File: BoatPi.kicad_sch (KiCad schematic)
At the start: 39 parts, among them J1 1432431, J2 1436987, J3 USB3_A_Stacked, J4 JAE_SIM_Card_SF72S006, J5 MDT420M01002, J6 G45A19071083HR, J7 1436987, J8 1432431, U1 SIM7600E-H, U2 PC817, U3 PC817, U4 PC817, U5 PC817, U6 PC817, U7 PC817, U8 PC817, U9 PC817

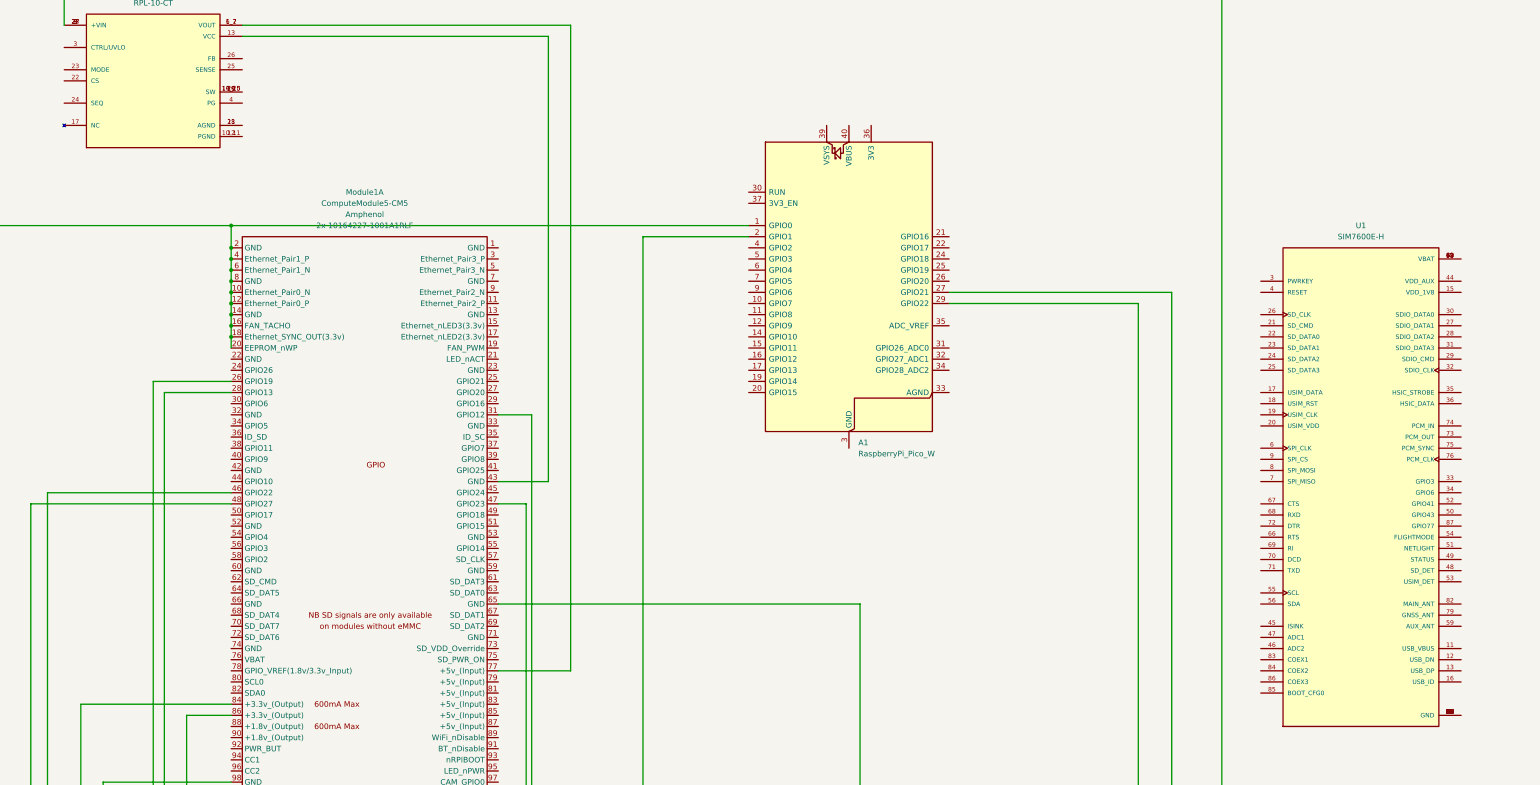
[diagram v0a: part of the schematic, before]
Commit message: Test Change
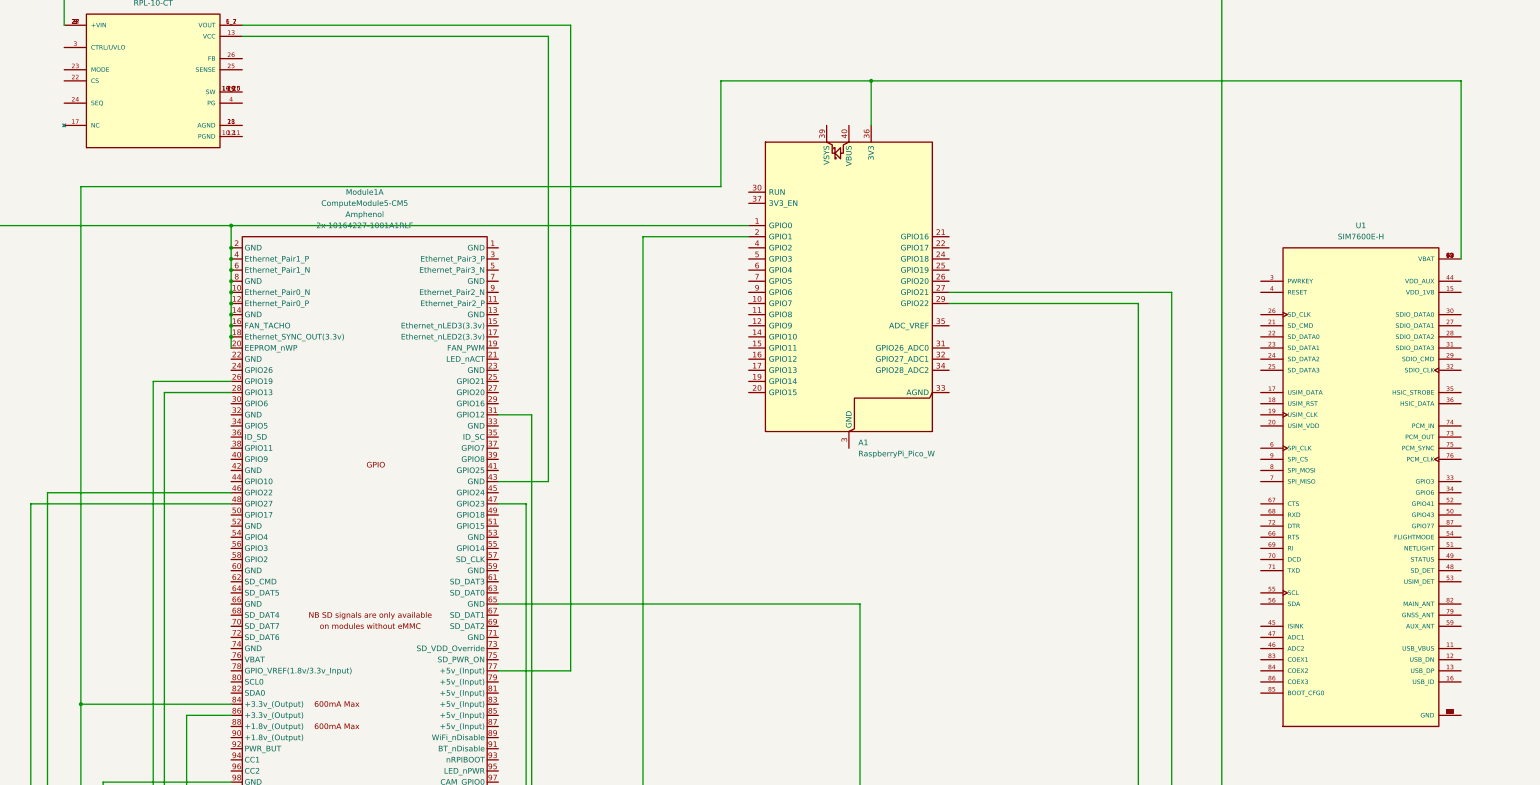
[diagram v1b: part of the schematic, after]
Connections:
- net at Module1.84 (+3.3v_(Output)), R11.1, R13.1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: now also A1.36 (3V3), U1.38 (VBAT), U1.39 (VBAT), U1.62 (VBAT), U1.63 (VBAT)
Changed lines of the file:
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@@
+	)
+	(junction
+		(at 39.37 274.32)
+		(diameter 0)
+		(color 0 0 0 0)
 	)
 	(junction
@@
 	)
 	(junction
+		(at 219.71 132.08)
+		(diameter 0)
+		(color 0 0 0 0)
+	)
+	(junction
 		(at 19.05 368.3)
 		(diameter 0)
@@
 	(wire
 		(pts
+			(xy 39.37 274.32) (xy 39.37 156.21)
+		)
+		(stroke
+			(width 0)
+			(type default)
+		)
+	)
+	(wire
+		(pts
 			(xy 217.17 330.2) (xy 217.17 331.47)
 		)
@@
 	(wire
 		(pts
+			(xy 39.37 156.21) (xy 185.42 156.21)
+		)
+		(stroke
+			(width 0)
+			(type default)
+		)
+	)
+	(wire
+		(pts
 			(xy 76.2 119.38) (xy 151.13 119.38)
 		)
@@
 	(wire
 		(pts
+			(xy 219.71 132.08) (xy 354.33 132.08)
+		)
+		(stroke
+			(width 0)
+			(type default)
+		)
+	)
+	(wire
+		(pts
 			(xy 177.8 372.11) (xy 177.8 328.93)
 		)
@@
 	(wire
 		(pts
+			(xy 185.42 132.08) (xy 219.71 132.08)
+		)
+		(stroke
+			(width 0)
+			(type default)
+		)
+	)
+	(wire
+		(pts
 			(xy 24.13 401.32) (xy 39.37 401.32)
 		)
@@
 	(wire
 		(pts
+			(xy 185.42 156.21) (xy 185.42 132.08)
+		)
+		(stroke
+			(width 0)
+			(type default)
+		)
+	)
+	(wire
+		(pts
 			(xy 77.47 354.33) (xy 58.42 354.33)
 		)
@@
 	(wire
 		(pts
+			(xy 354.33 172.72) (xy 354.33 132.08)
+		)
+		(stroke
+			(width 0)
+			(type default)
+		)
+	)
+	(wire
+		(pts
 			(xy 146.05 223.52) (xy 134.62 223.52)
 		)
@@
 		)
 		(stroke
+			(width 0)
+			(type default)
+		)
+	)
+	(wire
+		(pts
+			(xy 219.71 132.08) (xy 219.71 142.24)
+		)
+		(stroke

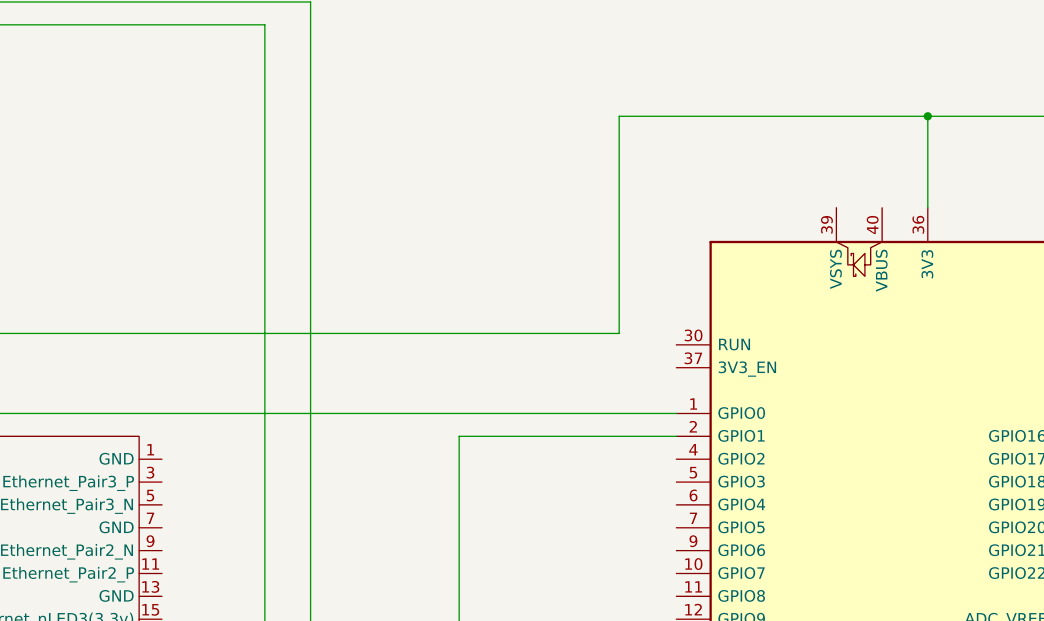
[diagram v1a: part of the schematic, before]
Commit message: New Test
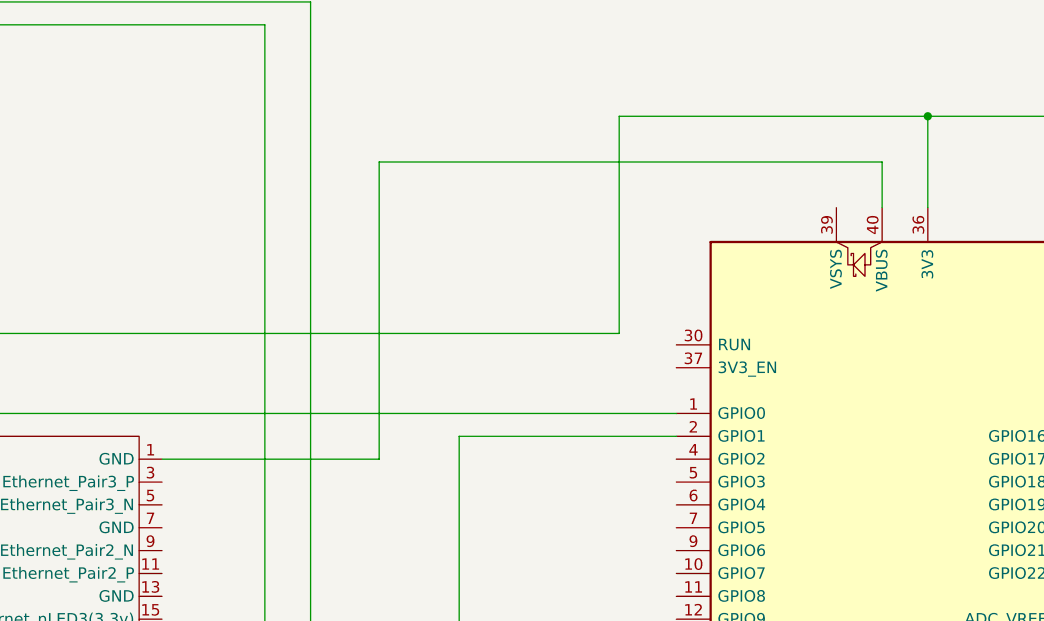
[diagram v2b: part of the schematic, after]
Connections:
- net at A1.40 (VBUS): now also Module1.1 (GND)
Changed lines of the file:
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@@
+	(wire
+		(pts
+			(xy 158.75 137.16) (xy 214.63 137.16)
+		)
+		(stroke
+			(width 0)
+			(type default)
+		)
+	)
 	(wire
 		(pts
@@
 	(wire
 		(pts
+			(xy 158.75 170.18) (xy 158.75 137.16)
+		)
+		(stroke
+			(width 0)
+			(type default)
+		)
+	)
+	(wire
+		(pts
 			(xy 55.88 200.66) (xy 55.88 332.74)
 		)
@@
 	(wire
 		(pts
+			(xy 214.63 137.16) (xy 214.63 142.24)
+		)
+		(stroke
+			(width 0)
+			(type default)
+		)
+	)
+	(wire
+		(pts
 			(xy 120.65 392.43) (xy 139.7 392.43)
 		)
@@
 		)
 		(stroke
+			(width 0)
+			(type default)
+		)
+	)
+	(wire
+		(pts
+			(xy 134.62 170.18) (xy 158.75 170.18)
+		)
+		(stroke
